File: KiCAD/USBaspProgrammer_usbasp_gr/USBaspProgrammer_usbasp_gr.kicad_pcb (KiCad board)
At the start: 2 copper layers, 20 parts, among them IC1 ATmega88-20PU, J3 Jumper_2_Bridged, K4 USB_A, Q2 12MHz

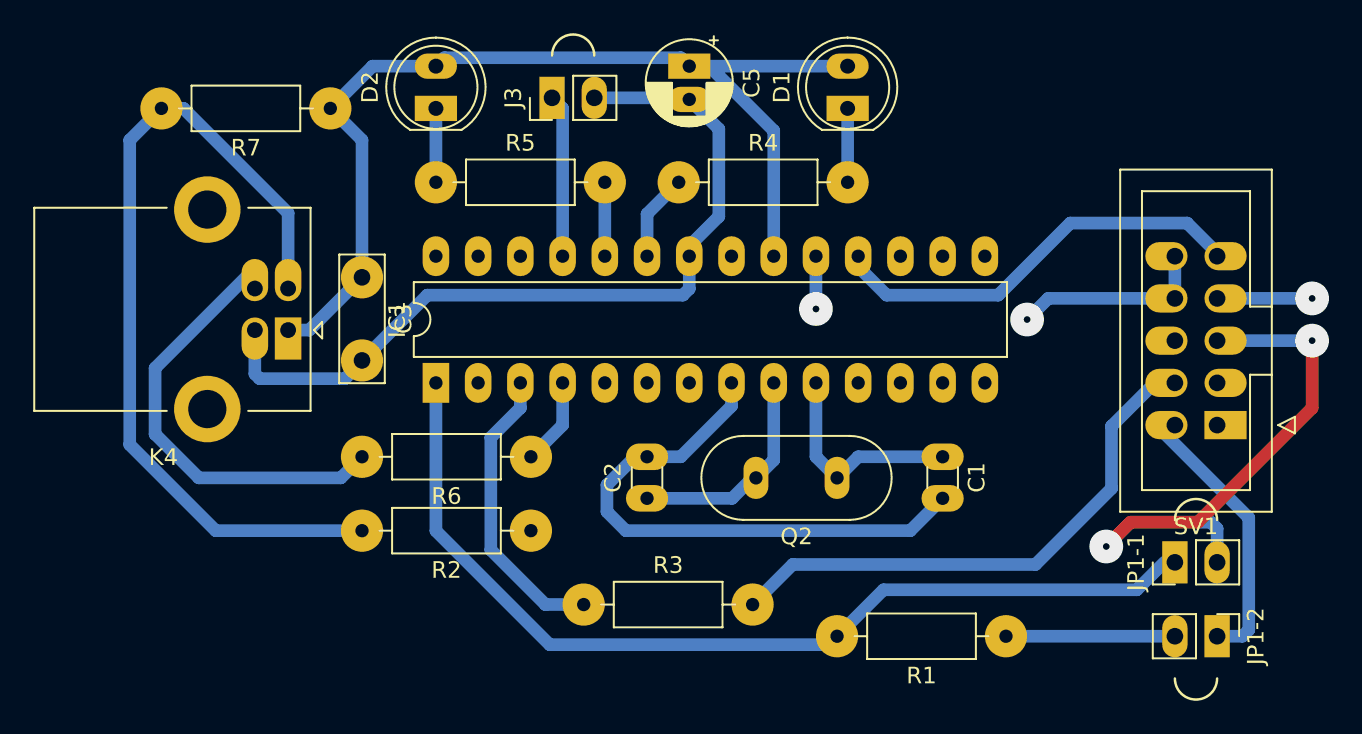
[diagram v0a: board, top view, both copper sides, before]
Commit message: kicad 6
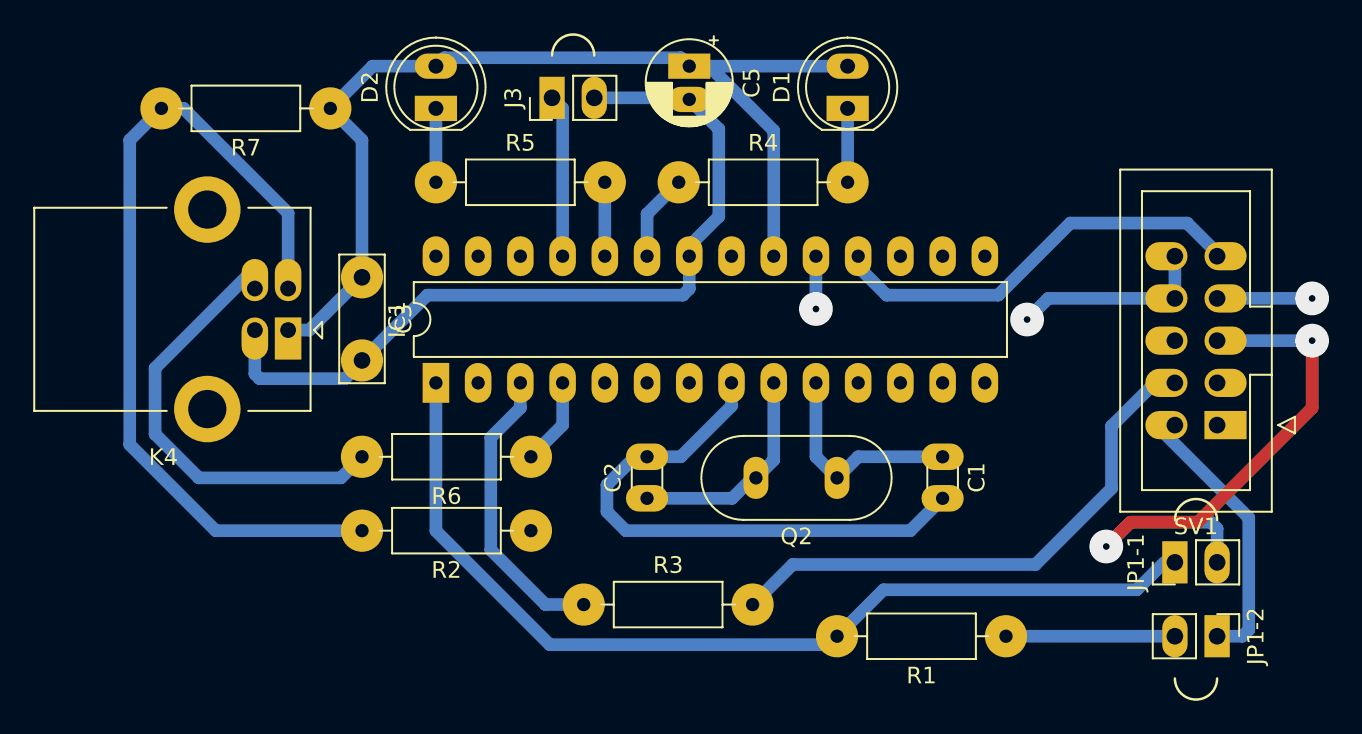
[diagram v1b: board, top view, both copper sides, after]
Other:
- net class Default removed
